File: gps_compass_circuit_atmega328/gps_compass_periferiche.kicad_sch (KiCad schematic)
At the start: 6 parts

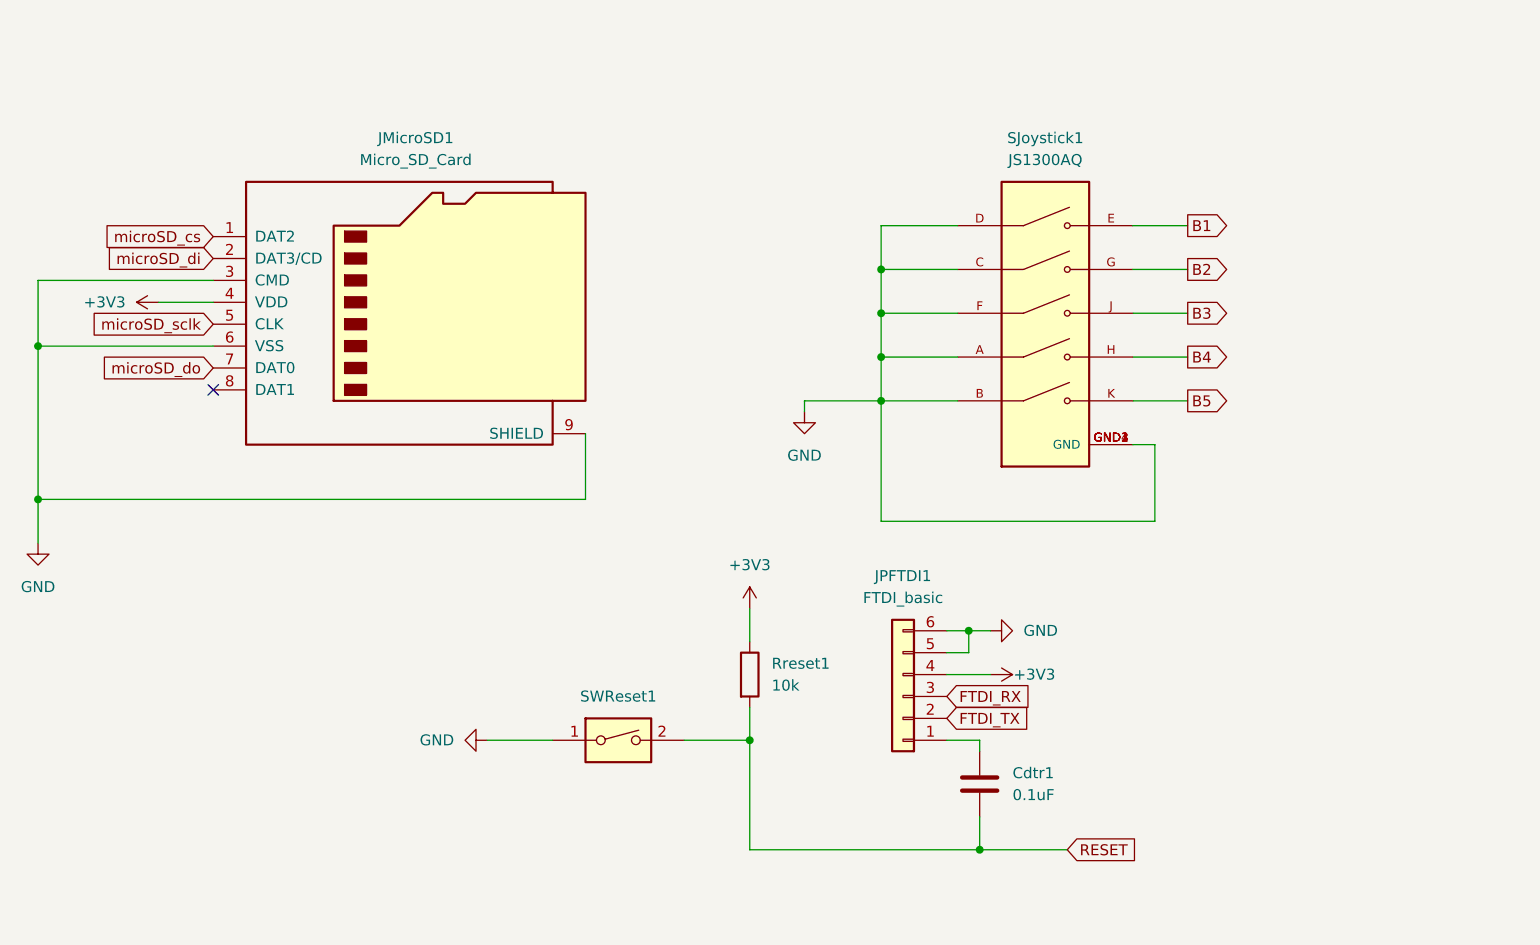
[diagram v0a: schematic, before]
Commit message: upd circuit
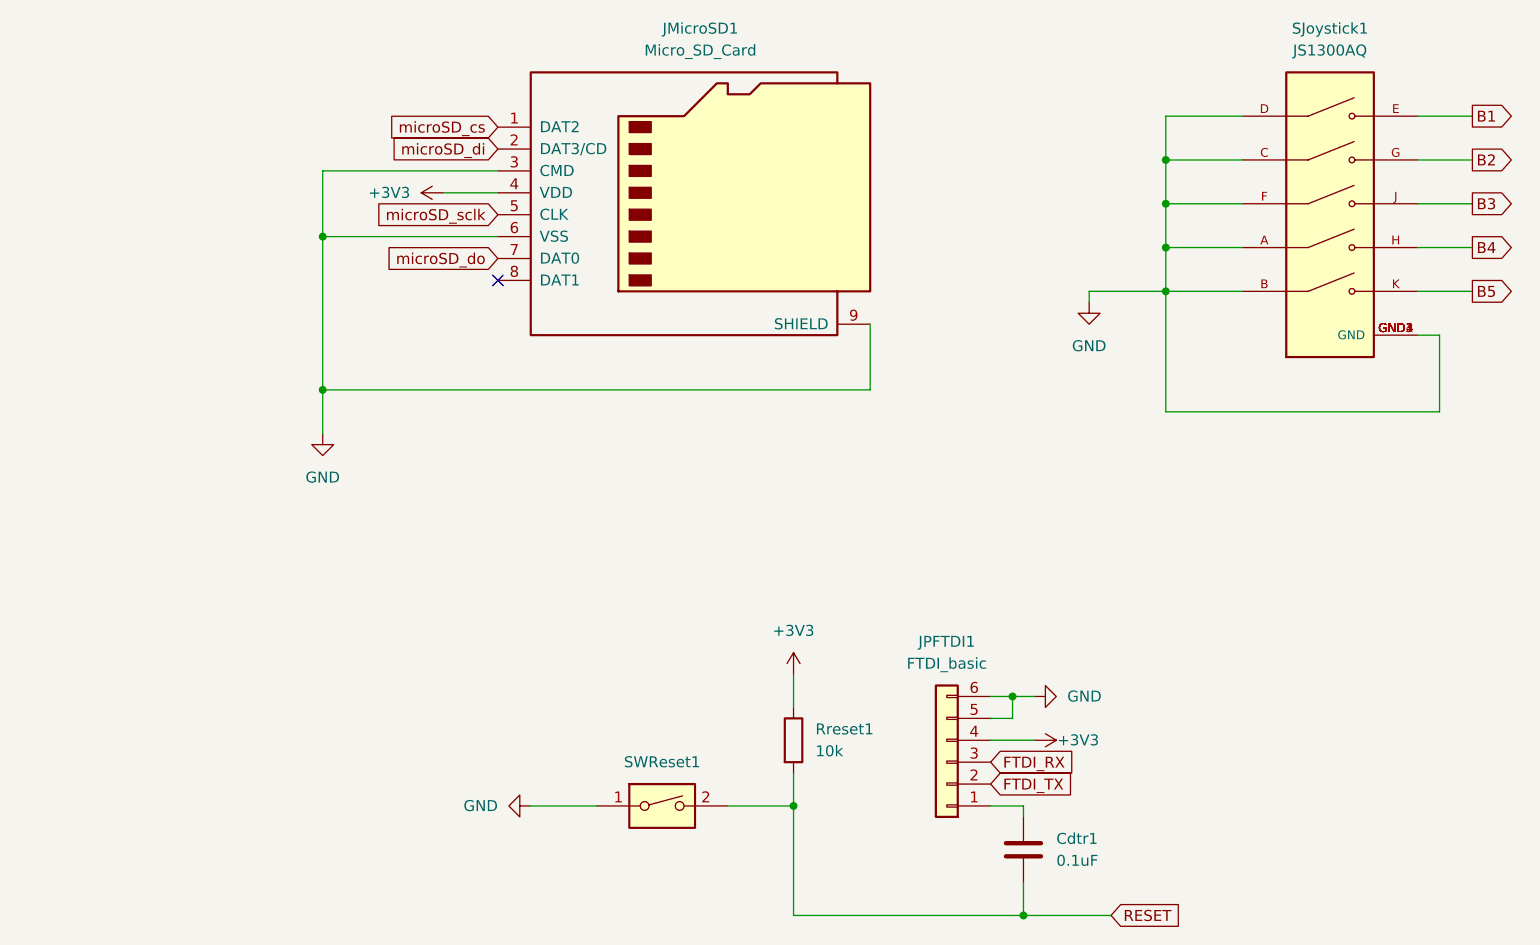
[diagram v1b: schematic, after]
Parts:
- SWReset1: footprint Button_Switch_SMD:SW_SPST_Omron_B3FS-101xP -> Button_Switch_THT:SW_PUSH_6mm
